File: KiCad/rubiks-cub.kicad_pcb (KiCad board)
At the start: 2 copper layers, 46 parts, among them J1 USB_B_Mini, J10 Conn_01x03_Pin, J11 Conn_01x03_Pin, J12 Conn_01x03_Pin, J13 Conn_01x01_Pin, J14 Conn_01x01_Pin, J15 Conn_01x01_Pin, J2 Conn_01x04_Pin, J3 Conn_01x04_Pin, J4 Conn_01x04_Pin, J5 Jack-DC, J6 Conn_01x01_Pin, J7 Conn_01x03_Pin, J8 Conn_01x03_Pin, J9 Conn_01x04_Pin, SW1 SW_SPDT, SW2 SW_Push, U1 STM32F401RETx, U2 AMS1117-3.3, Y1 16MHz

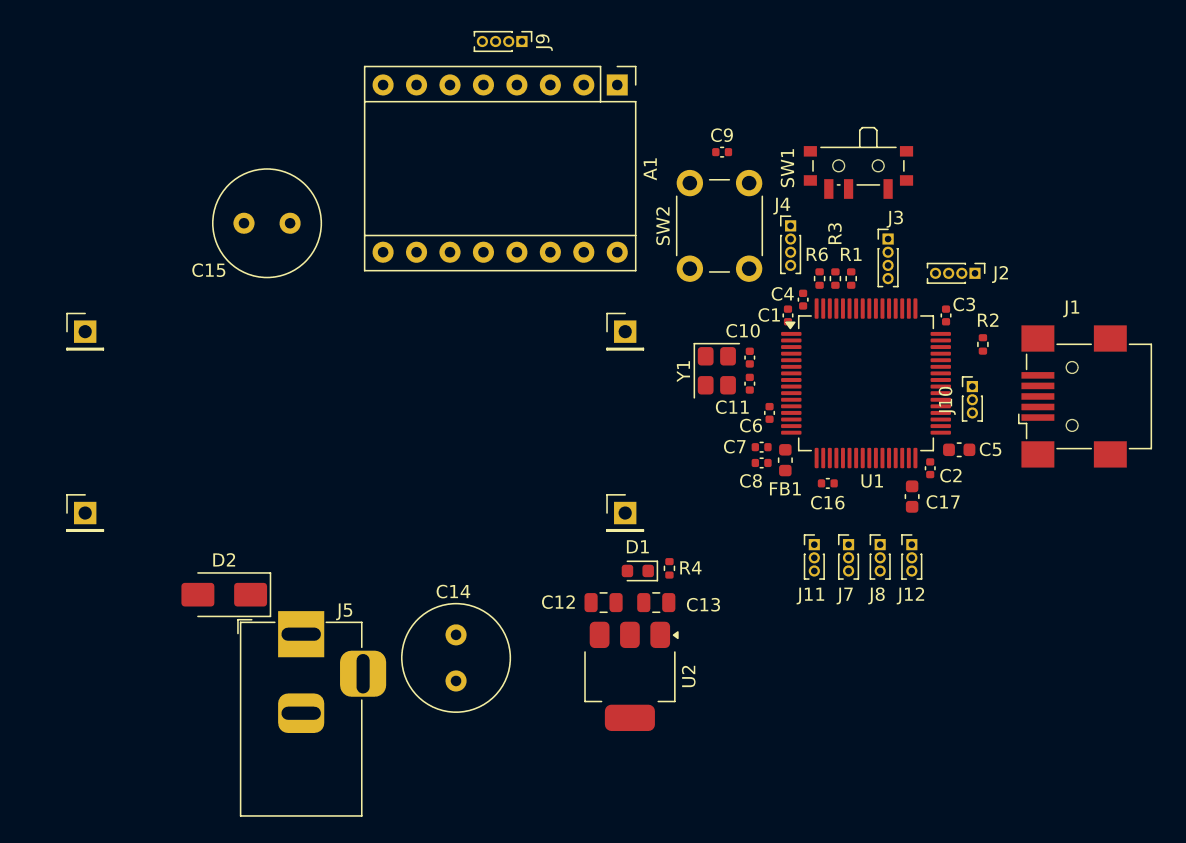
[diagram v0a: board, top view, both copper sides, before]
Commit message: pcb design
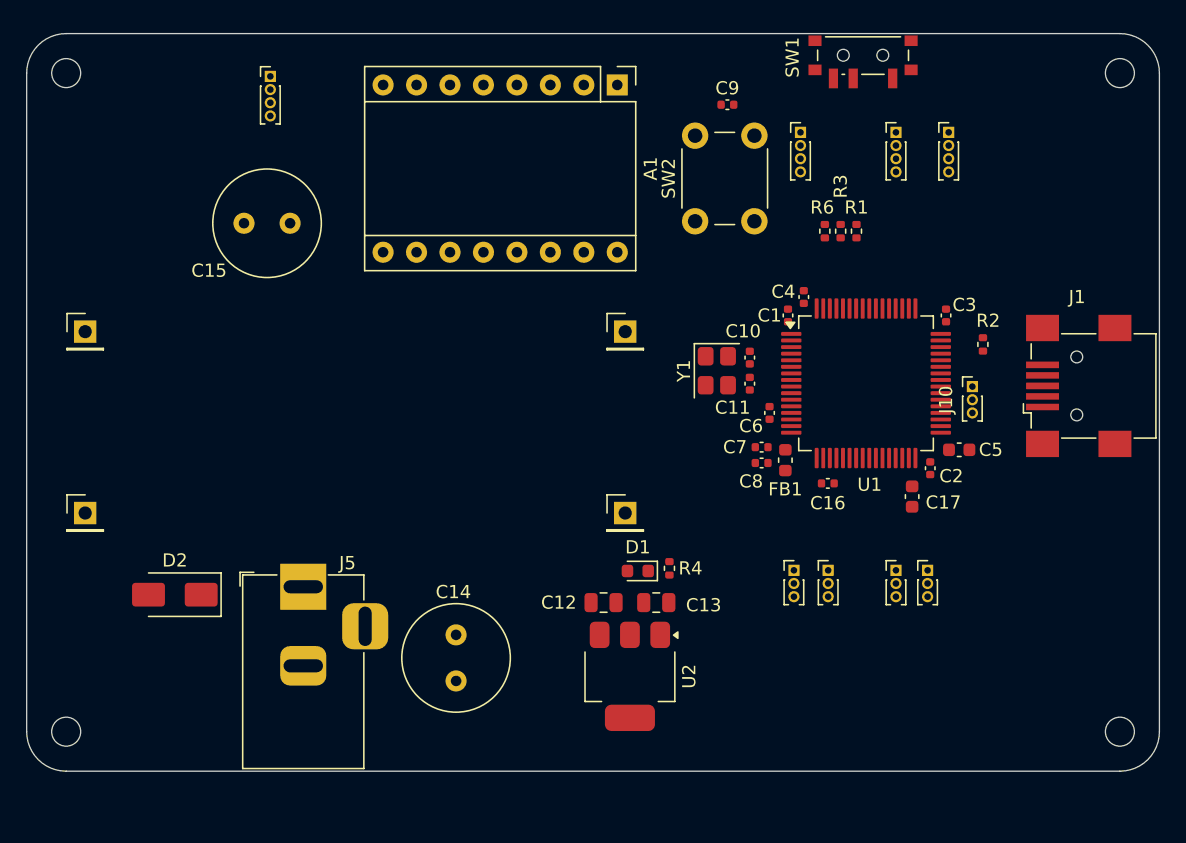
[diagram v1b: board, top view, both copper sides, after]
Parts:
- added H1: MountingHole, MountingHole:MountingHole_2.2mm_M2, F.Cu at (62.0, 95.0)
- added H2: MountingHole, MountingHole:MountingHole_2.2mm_M2, F.Cu at (142.0, 95.0)
- added H3: MountingHole, MountingHole:MountingHole_2.2mm_M2, F.Cu at (62.0, 145.0)
- added H4: MountingHole, MountingHole:MountingHole_2.2mm_M2, F.Cu at (142.0, 145.0)
- moved J9 19.3 mm to (77.5, 95.2), turned to 0 degrees
- moved J2 10.9 mm to (129.0, 99.5), turned to 0 degrees
- moved SW1 8.40 mm to (122.5, 94.0)
- moved J3 8.12 mm to (125.0, 99.5)
- moved J4 7.14 mm to (117.8, 99.5)
- moved D2 3.75 mm to (70.2, 134.6)
- moved C9 3.62 mm to (112.2, 97.4)
- moved R1 3.62 mm to (122.0, 107.0)
- moved SW2 3.62 mm to (109.8, 106.2)
- moved R3 3.62 mm to (120.8, 107.0)
- moved R6 3.62 mm to (119.6, 107.0)
- moved J5 3.60 mm to (80.0, 134.0)
- moved J7 2.49 mm to (119.8, 132.8)
- moved J11 2.49 mm to (117.2, 132.8)
- moved J12 2.29 mm to (127.4, 132.8)
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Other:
- board outline added: 86 x 56 mm
